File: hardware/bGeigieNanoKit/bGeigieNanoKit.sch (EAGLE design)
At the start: 35 parts, among them T1 2SC1815

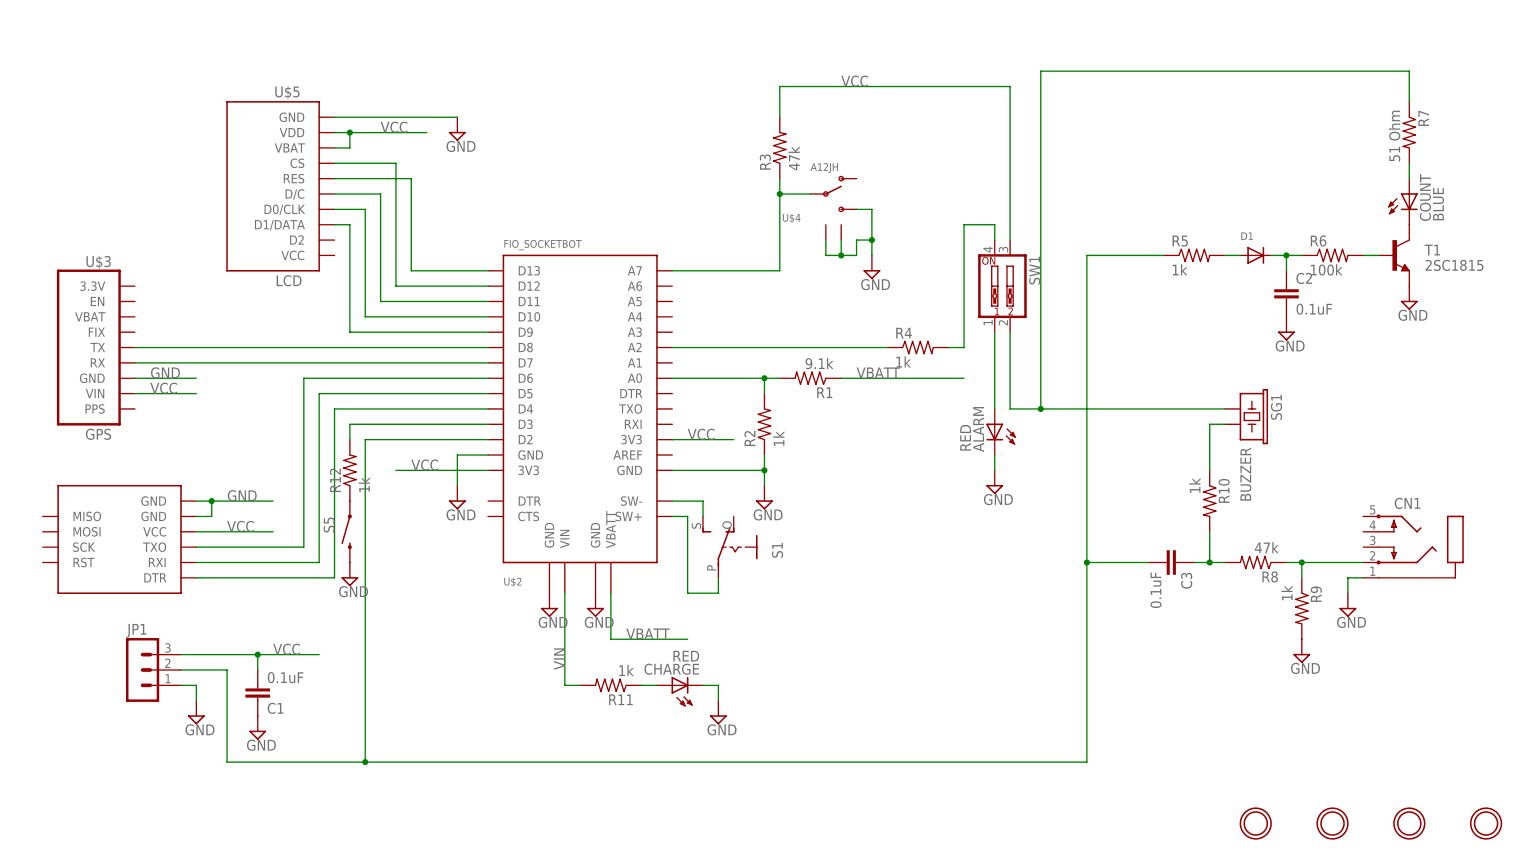
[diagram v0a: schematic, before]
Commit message: rc1
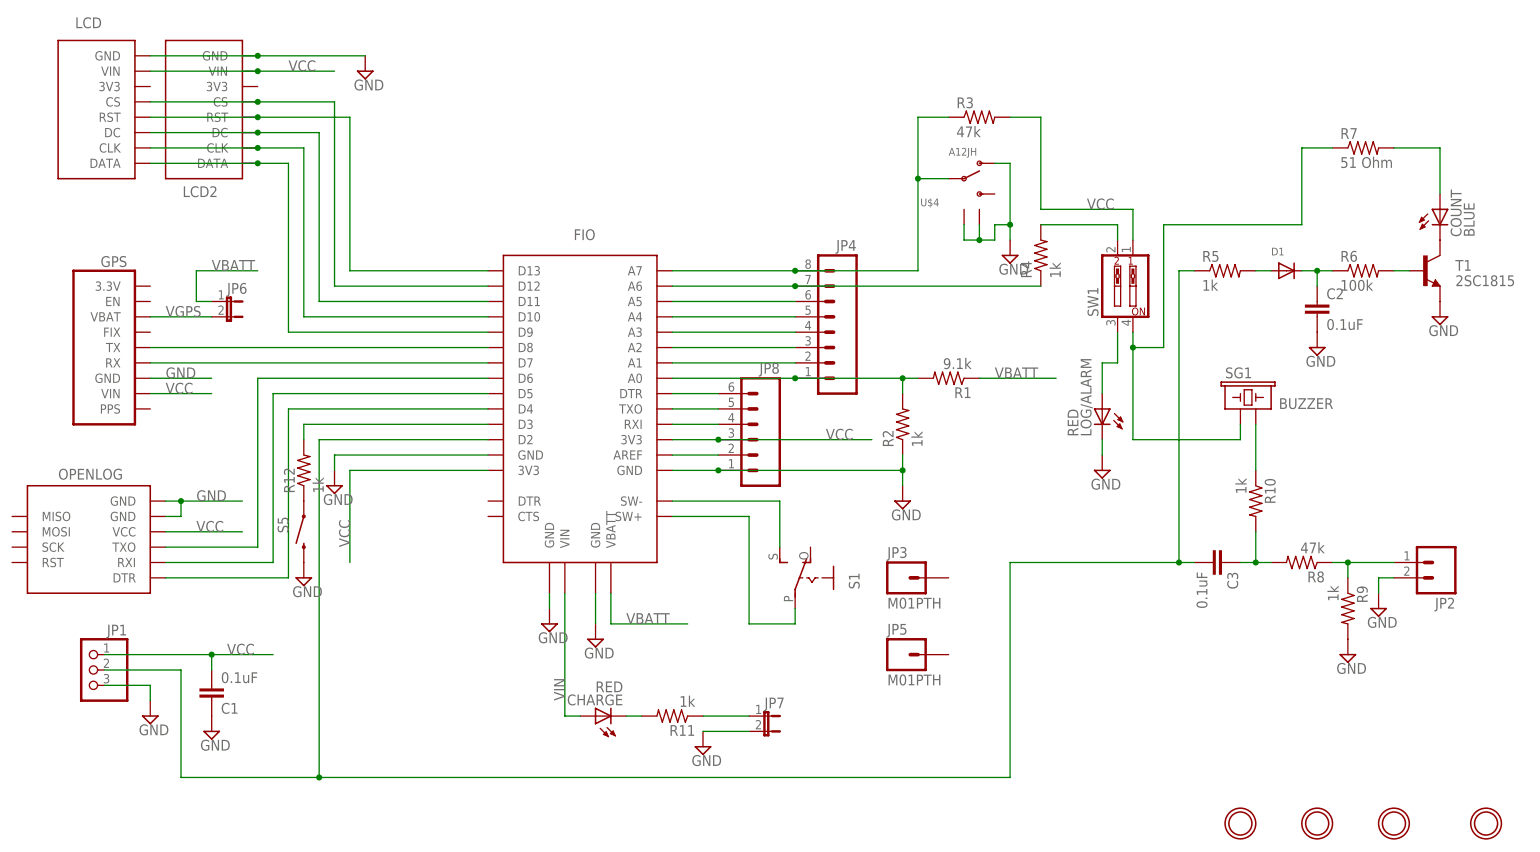
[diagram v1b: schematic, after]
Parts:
- removed ALARM: RED, adafruit:LED3MM
- removed CN1: (no value), microbuilder:AUDIO_STEREOJACK
- removed U$1: OPENLOG, open_hw_sockets:OPENLOG
- removed U$2: FIO_SOCKETBOT, open_hw_sockets:FIO_SOCKETBOT
- removed U$3: GPS, open_hw_sockets:ULTIMATE_GPSTOP
- removed U$5: LCD, open_hw_sockets:SSD1306_128X64_LCD_MIN
- added FIO: FIO_SOCKETBOT, open_hw_sockets:FIO_SOCKETBOT
- added GPS: ULTIMATE_GPSTOP, open_hw_sockets:ULTIMATE_GPSTOP
- added JP2: (no value), SparkFun:M02PTH
- added JP3, JP5: M01PTH, SparkFun:M01PTH
- added JP4: (no value), SparkFun:M081X08
- added JP6: (no value), SparkFun:JUMPER-2SMD-NO
- added JP7: (no value), microbuilder:JUMPER2
- added JP8: (no value), SparkFun:M06SIP
- added LCD: SSD1306_128X64_V2_LCD1.3IN_TOP, open_hw_sockets:SSD1306_128X64_V2_LCD1.3IN_TOP
- added LCD2: SSD1306_128X64_V2_LCD0.96IN_MIN, open_hw_sockets:SSD1306_128X64_V2_LCD0.96IN_MIN
- added LOG/ALARM: RED, adafruit:LED3MM
- added OPENLOG: OPENLOG, open_hw_sockets:OPENLOG
- JP1: device con-lstb:MA03-1 -> pinhead:PINHD-1X3/90
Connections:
- new net N$31: CHARGE.C, R11.2
- new net N$32: R7.1, SG1.1, SW1.4
- new net N$33: FIO.A4, JP4.5
- new net N$34: FIO.A3, JP4.4
- new net N$35: FIO.A2, JP4.3
- new net N$36: FIO.A1, JP4.2
- new net N$37: FIO.DTR@1, JP8.6
- new net N$38: FIO.TXO, JP8.5
- new net N$39: FIO.RXI, JP8.4
- new net N$40: FIO.AREF, JP8.2
- new net VGPS: GPS.VBAT, JP6.2
- net GND: now also FIO.GND@1, FIO.GND@2, FIO.GND@3, FIO.GND@4, GPS.GND, JP1.3, JP2.2, JP7.2, JP8.1, LCD.GND, LCD2.GND, LOG/ALARM.C, OPENLOG.GND@1, OPENLOG.GND@2, U$4.P$1; no longer ALARM.C, CHARGE.C, CN1.1, JP1.1, U$1.GND@1, U$1.GND@2, U$2.GND@1, U$2.GND@2, U$2.GND@3, U$2.GND@4, U$3.GND, U$4.P$3, U$5.GND
- net N$1: now also FIO.D9, LCD.DATA, LCD2.DATA; no longer U$2.D9, U$5.D1/DATA
- net N$10: now also FIO.D4, OPENLOG.DTR; no longer U$1.DTR, U$2.D4
- net N$11: now also FIO.A0, JP4.1; no longer U$2.A0
- net N$12: now also FIO.SW+; no longer U$2.SW+
- net N$13: now also FIO.SW-; no longer U$2.SW-
- net N$14: now also FIO.A7, JP4.8; no longer U$2.A7
- net N$15: now also FIO.A6, JP4.7; no longer U$2.A2
- net N$16: now also LOG/ALARM.A, SW1.3; no longer ALARM.A, SW1.1
- net N$17: now also SW1.2; no longer SW1.4
- net N$18: now also FIO.D2; no longer U$2.D2
- net N$2: now also FIO.D10, LCD.CLK, LCD2.CLK; no longer U$2.D10, U$5.D0/CLK
- net N$21: now also FIO.A5, JP4.6; no longer R7.1, SG1.1, SW1.2
- net N$25: now also JP2.1; no longer CN1.2
- net N$29: now also JP7.1; no longer CHARGE.A
- net N$3: now also FIO.D11, LCD.DC, LCD2.DC; no longer U$2.D11, U$5.D/C
- net N$30: now also FIO.D3; no longer U$2.D3
- net N$4: now also FIO.D12, LCD.CS, LCD2.CS; no longer U$2.D12, U$5.CS
- net N$5: now also FIO.D13, LCD.RST, LCD2.RST; no longer U$2.D13, U$5.RES
- net N$6: now also FIO.D8, GPS.TX; no longer U$2.D8, U$3.TX
- net N$7: now also FIO.D7, GPS.RX; no longer U$2.D7, U$3.RX
- net N$8: now also FIO.D6, OPENLOG.TXO; no longer U$1.TXO, U$2.D6
- net N$9: now also FIO.D5, OPENLOG.RXI; no longer U$1.RXI, U$2.D5
- net VBATT: now also FIO.VBATT, JP6.1; no longer U$2.VBATT
- net VCC: now also FIO.3V3@1, FIO.3V3@2, GPS.VIN, JP1.1, JP8.3, LCD.VIN, LCD2.VIN, OPENLOG.VCC, SW1.1; no longer JP1.3, SW1.3, U$1.VCC, U$2.3V3@1, U$2.3V3@2, U$3.VIN, U$5.VBAT, U$5.VDD
- net VIN: now also CHARGE.A, FIO.VIN; no longer R11.2, U$2.VIN
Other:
- moved on the sheet: C1, C2, C3, CHARGE, COUNT, D1, R1, R10, R11, R12, R2, R3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
